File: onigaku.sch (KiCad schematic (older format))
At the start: 312 parts, among them J1 MJ-4PP-9, J2 MJ-4PP-9, U1 Elite-C, U2 Elite-C

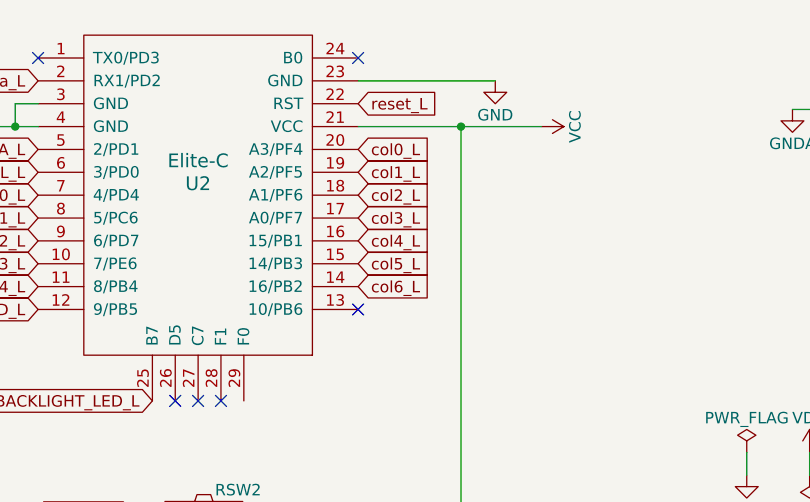
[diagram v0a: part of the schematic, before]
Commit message: wiring up oleds and trs. starting left side
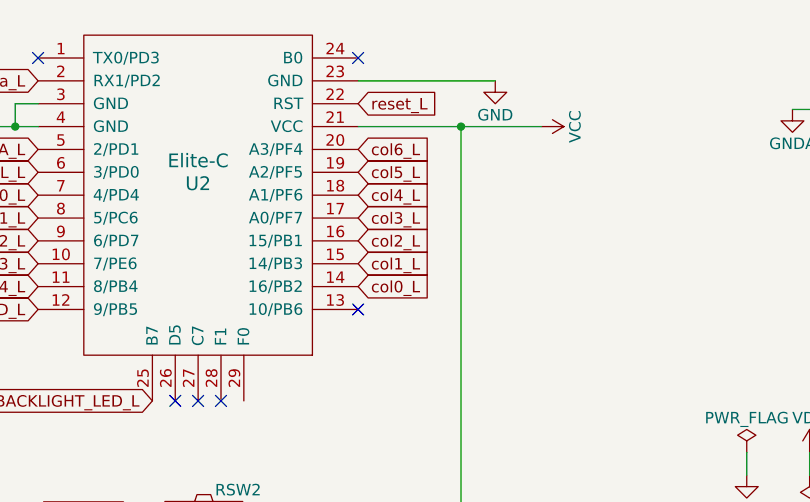
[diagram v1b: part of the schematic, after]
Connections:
- net col0_L: now also U2.14 (16/PB2); no longer U2.20 (A3/PF4)
- net col1_L: now also U2.15 (14/PB3); no longer U2.19 (A2/PF5)
- net col2_L: now also U2.16 (15/PB1); no longer U2.18 (A1/PF6)
- net col4_L: now also U2.18 (A1/PF6); no longer U2.16 (15/PB1)
- net col5_L: now also U2.19 (A2/PF5); no longer U2.15 (14/PB3)
- net col6_L: now also U2.20 (A3/PF4); no longer U2.14 (16/PB2)
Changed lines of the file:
@@
 Text GLabel 9900 2025 0    50   Input ~ 0
 row4_L
-Text GLabel 11300 1425 2    50   Input ~ 0
+Text GLabel 11300 2025 2    50   Input ~ 0
 col0_L
-Text GLabel 11300 1525 2    50   Input ~ 0
+Text GLabel 11300 1925 2    50   Input ~ 0
 col1_L
-Text GLabel 11300 1625 2    50   Input ~ 0
+Text GLabel 11300 1825 2    50   Input ~ 0
 col2_L
 Text GLabel 11300 1725 2    50   Input ~ 0
 col3_L
-Text GLabel 11300 1825 2    50   Input ~ 0
+Text GLabel 11300 1625 2    50   Input ~ 0
 col4_L
-Text GLabel 11300 2025 2    50   Input ~ 0
+Text GLabel 11300 1425 2    50   Input ~ 0
 col6_L
 Wire Wire Line
@@
 	17300 5150 17300 6150
 Connection ~ 17300 5150
-Text GLabel 11300 1925 2    50   Input ~ 0
+Text GLabel 11300 1525 2    50   Input ~ 0
 col5_L
 Wire Wire Line
